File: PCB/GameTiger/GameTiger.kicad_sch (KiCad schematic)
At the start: 73 parts, among them J1 USB_C_Receptacle_USB2.0, J2 503398-1892, J3 LCD Display, J4 Speaker, Q3 DMG3415, U1 RP2040, U2 MCP73831-2-OT, U3 W25Q128JVSIQ, U4 PAM8302A, U5 AP2112K-3.3, U6 PCF8574TS, Y1 ABLS-12MHZ-B4-T

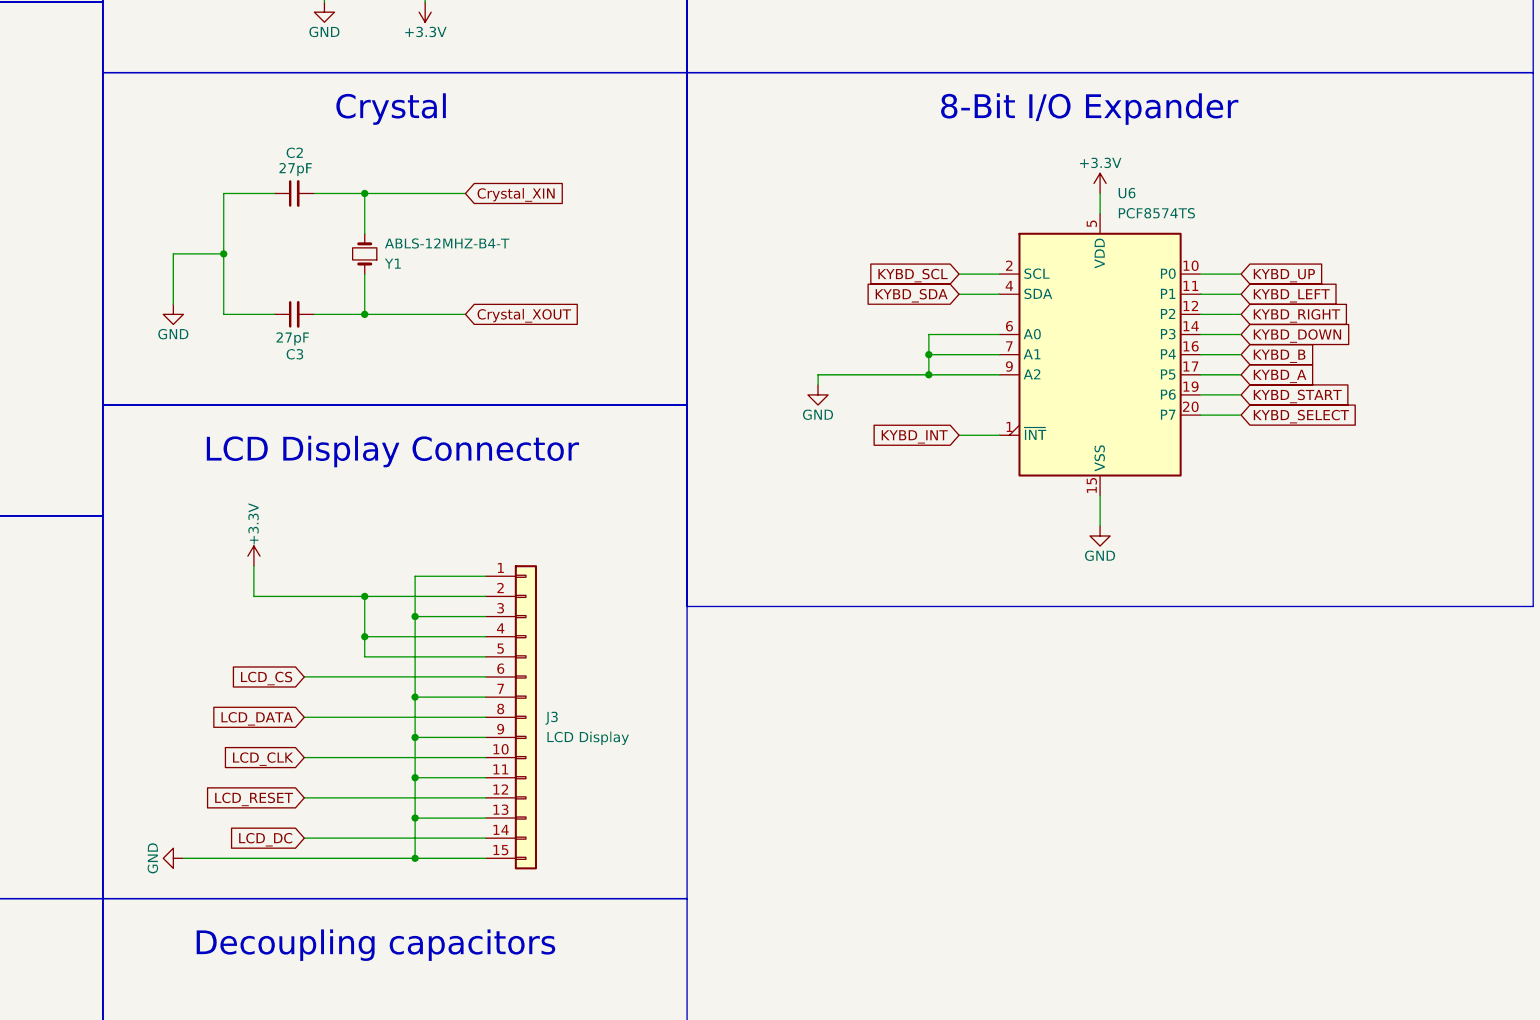
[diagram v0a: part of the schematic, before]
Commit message: Ready for uploading to JLCPCB
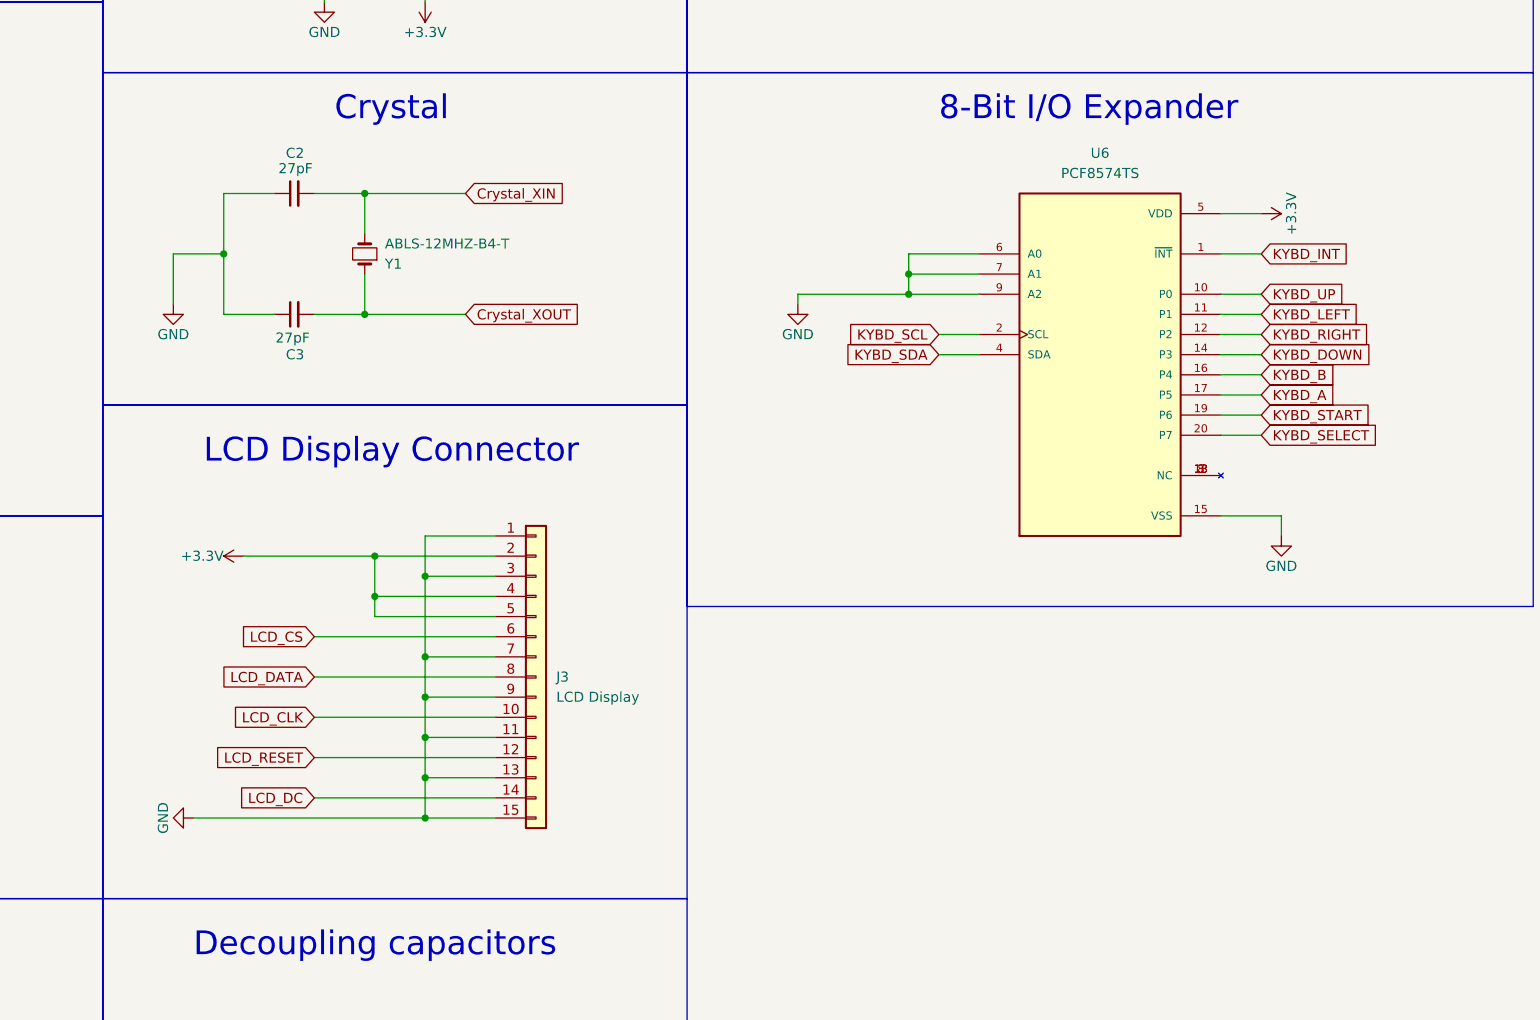
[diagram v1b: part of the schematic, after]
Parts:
- A1, B1, Down1, Left1, Right1, Up1: LCSC (none) -> C411882
- Boot1, Reset1: LCSC (none) -> C231329
- C1, C19, C22, C23, C4: LCSC (none) -> C1713
- C17, C18, C6, C9: LCSC (none) -> C14445
- C20, C21: LCSC (none) -> C61747
- D1: LCSC (none) -> C3018524
- D2: LCSC (none) -> C965791
- FB1, FB2: LCSC (none) -> C44838; Manuf. Part # BLM21AG102BH1D -> CBW201209U102T; Manufacturer Murata Electronics -> FH (Guangdong Fenghua Advanced Tech)
- J1: LCSC (none) -> C2988369
- J2: LCSC (none) -> C428492
- J3: LCSC (none) -> C262664; Manuf. Part # AFC07-S15FCA-00 -> AFC01-S15FCA-00
- Power1: LCSC (none) -> C221660
- Q3: LCSC (none) -> C96616
- R1, R5: LCSC (none) -> C11702
- R10, R12, R13, R16, R2, R6: LCSC (none) -> C25744
- R11, R14, R15: LCSC (none) -> C25905
- R3, R4: footprint Resistor_SMD:R_0402_1005Metric -> Resistor_SMD:R_0603_1608Metric; LCSC (none) -> C25190; Size 0402_1005Metric -> 0603_1608Metric
- R7: LCSC (none) -> C719176
- R8, R9: LCSC (none) -> C25076
- Select1, Start1: LCSC (none) -> C221678
- U1: LCSC (none) -> C2040
- U2: LCSC (none) -> C424093
- U3: LCSC (none) -> C113767
- U4: LCSC (none) -> C113367
- U5: LCSC (none) -> C51118
- U6: footprint Package_SO:SSOP-20_4.4x6.5mm_P0.65mm -> SOP65P640X150-20N; symbol Interface_Expansion:PCF8574TS -> PCF8574TS:PCF8574TS; A1_MIN (none) -> 0.0; A_MAX (none) -> 1.5; A_MIN (none) -> 1.5; A_NOM (none) -> 1.5; B_MAX (none) -> 0.32; B_MIN (none) -> 0.2; B_NOM (none) -> 0.26; D2_MAX (none) -> 0.0; D_MAX (none) -> 6.6; D_MIN (none) -> 6.4; D_NOM (none) -> 6.5; E1_MAX (none) -> 4.5; E1_MIN (none) -> 4.3; E1_NOM (none) -> 4.4; E2_MAX (none) -> 0.0; ENOM (none) -> 0.65; E_MAX (none) -> 6.6; E_MIN (none) -> 6.2; E_NOM (none) -> 6.4; LCSC (none) -> C57790; L_MAX (none) -> 0.75; L_MIN (none) -> 0.45; L_NOM (none) -> 0.6; MANUFACTURER (none) -> NXP; PARTREV (none) -> 5; PIN_COUNT (none) -> 20.0; STANDARD (none) -> IPC 7351B
- X1: LCSC (none) -> C295747
- Y1: LCSC (none) -> C2901718
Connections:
- net at U6.13 (NC): now also U6.18 (NC), U6.3 (NC), U6.8 (NC)
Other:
- moved on the sheet: J3
